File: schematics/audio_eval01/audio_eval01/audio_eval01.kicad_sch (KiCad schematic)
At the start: 2 parts, among them J1 Conn_01x08_Pin

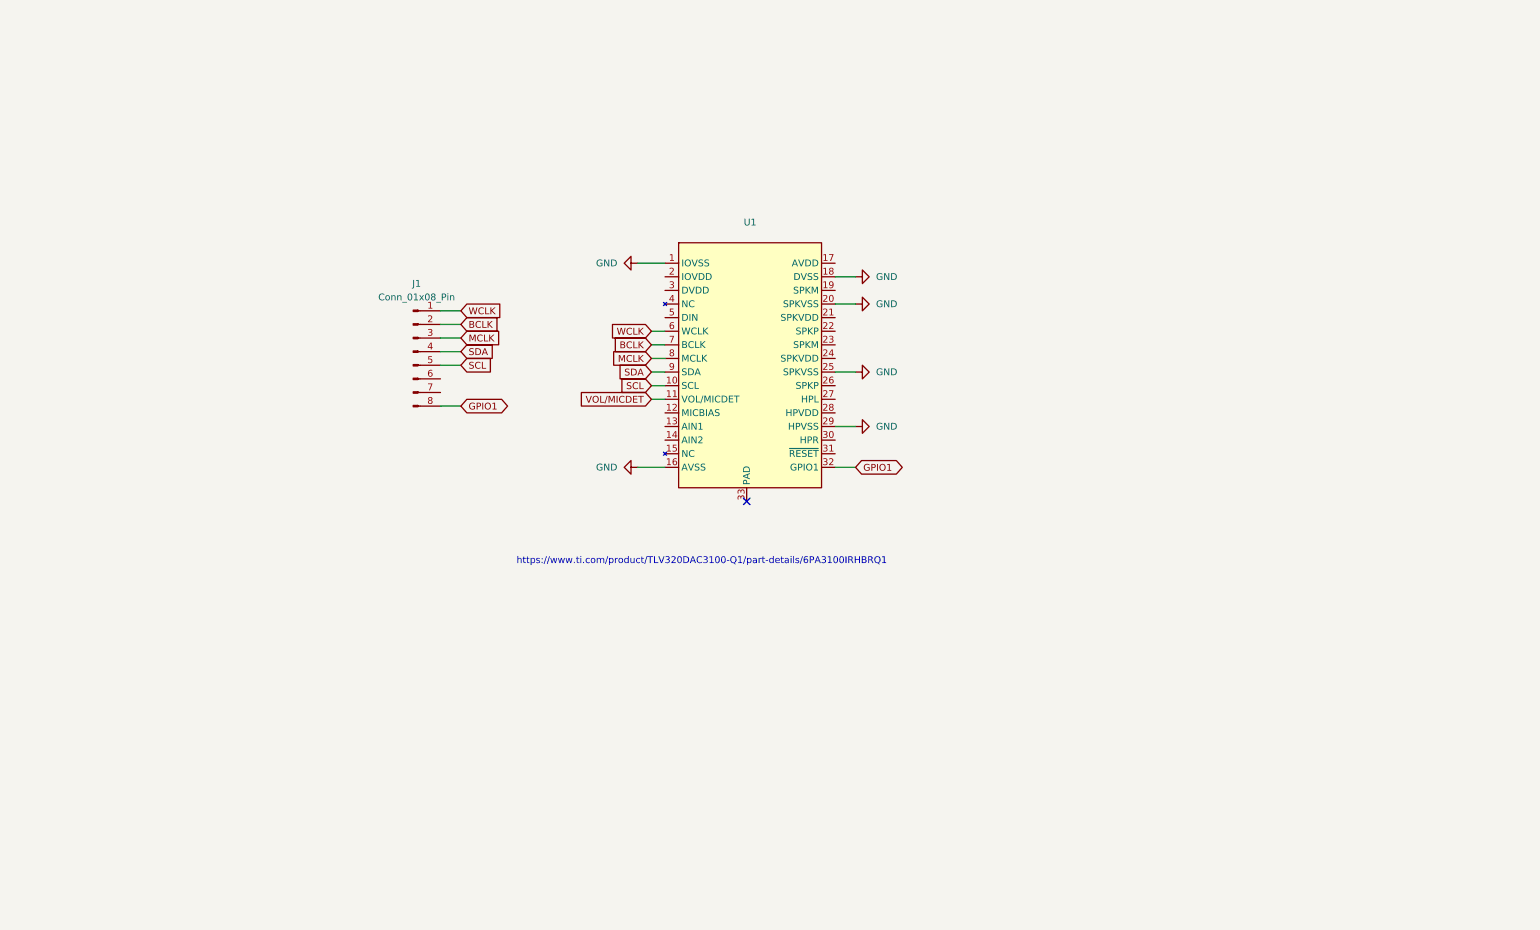
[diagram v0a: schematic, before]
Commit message: Audio evaluation board work.
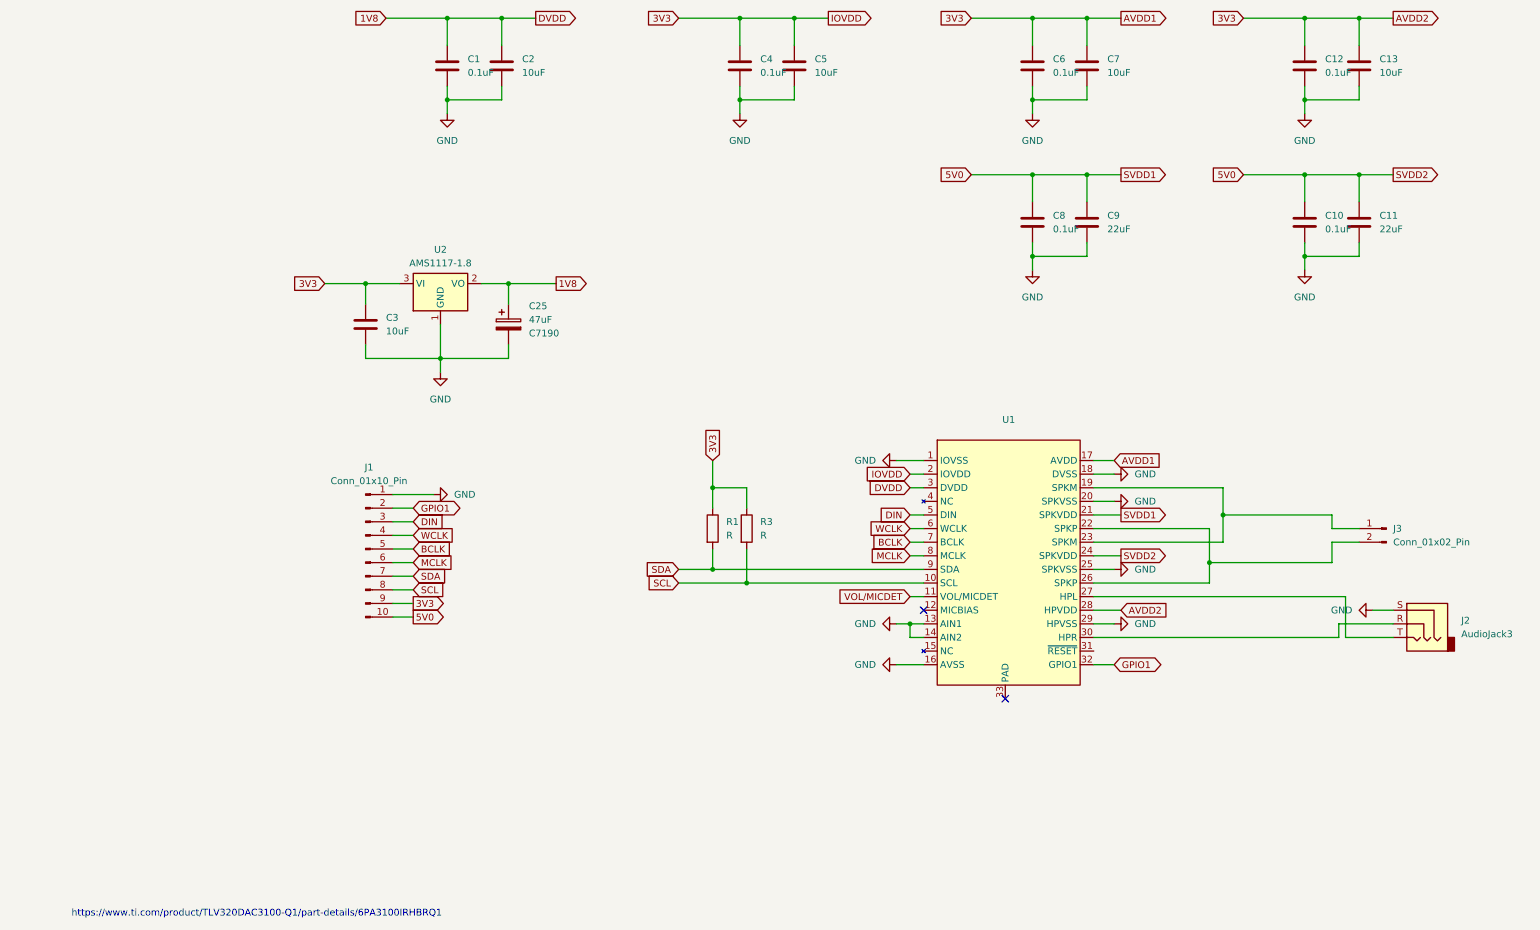
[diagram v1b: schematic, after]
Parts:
- added C1, C10, C12, C4, C6, C8: 0.1uF, Capacitor_SMD:C_0805_2012Metric_Pad1.18x1.45mm_HandSolder, symbol Device:C
- added C11, C9: 22uF, Capacitor_SMD:C_0805_2012Metric_Pad1.18x1.45mm_HandSolder, symbol Device:C
- added C13, C2, C3, C5, C7: 10uF, Capacitor_SMD:C_0805_2012Metric_Pad1.18x1.45mm_HandSolder, symbol Device:C
- added C25: 47uF, Capacitor_Tantalum_SMD:CP_EIA-3216-18_Kemet-A, symbol Device:C_Polarized
- added J2: AudioJack3, Connector_Audio:Jack_3.5mm_Switronic_ST-005-G_horizontal, symbol Connector_Audio:AudioJack3
- added J3: Conn_01x02_Pin, Connector_PinHeader_2.54mm:PinHeader_1x02_P2.54mm_Vertical, symbol Connector:Conn_01x02_Pin
- added R1, R3: R, Resistor_SMD:R_0805_2012Metric_Pad1.20x1.40mm_HandSolder, symbol Device:R
- added U2: AMS1117-1.8, Package_TO_SOT_SMD:SOT-223-3_TabPin2, symbol Regulator_Linear:AMS1117-1.8
- J1: value Conn_01x08_Pin -> Conn_01x10_Pin; footprint Connector_PinHeader_2.54mm:PinHeader_1x08_P2.54mm_Vertical -> Connector_PinHeader_2.54mm:PinHeader_1x10_P2.54mm_Vertical; symbol Connector:Conn_01x08_Pin -> Connector:Conn_01x10_Pin
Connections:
- net BCLK: now also J1.5 (Pin_5); no longer J1.2 (Pin_2)
- net GND: now also J1.1 (Pin_1), U1.13 (AIN1), U1.14 (AIN2), C1.2, C10.2, C11.2, C12.2, C13.2, C2.2, C25.2, C3.2, C4.2, C5.2, C6.2, C7.2, C8.2, C9.2, J2.S, U2.1 (GND)
- net GPIO1: now also J1.2 (Pin_2); no longer J1.8 (Pin_8)
- net MCLK: now also J1.6 (Pin_6); no longer J1.3 (Pin_3)
- net SCL: now also J1.8 (Pin_8), R3.2; no longer J1.5 (Pin_5)
- net SDA: now also J1.7 (Pin_7), R1.2; no longer J1.4 (Pin_4)
- net WCLK: now also J1.4 (Pin_4); no longer J1.1 (Pin_1)
- net 3V3: now reaches U1.17 (AVDD)
- net 3V3: now also J1.9 (Pin_9), U1.2 (IOVDD), U1.28 (HPVDD), C12.1, C13.1, C3.1, C4.1, C5.1, C6.1, C7.1, R1.1, R3.1, U2.3 (VI)
- net at U1.19 (SPKM): now also U1.23 (SPKM), J3.1 (Pin_1)
- net 5V0: now reaches U1.21 (SPKVDD)
- net 5V0: now also J1.10 (Pin_10), U1.24 (SPKVDD), C10.1, C11.1, C8.1, C9.1
- net at U1.22 (SPKP): now also U1.26 (SPKP), J3.2 (Pin_2)
- net at U1.27 (HPL): now also J2.T
- net 1V8: now reaches U1.3 (DVDD)
- net 1V8: now also C1.1, C2.1, C25.1, U2.2 (VO)
- net at U1.30 (HPR): now also J2.R
- net DIN: now reaches U1.5 (DIN)
- net DIN: now also J1.3 (Pin_3)
- no-connect marks 1 -> 2
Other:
- moved on the sheet: U1
